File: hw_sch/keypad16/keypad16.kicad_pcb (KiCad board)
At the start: 2 copper layers, 70 x 100 mm, 174 parts, among them J1 Conn_01x04_Pin, J2 Conn_01x10_Pin, SW1 SW_Push, U1 MSP430FR2633IDAR, U2 TS5A23159RSE, U3 TS5A23159RSE, U4 TS5A23159RSE, U5 TS5A23159RSE, Y1 32.768KHz

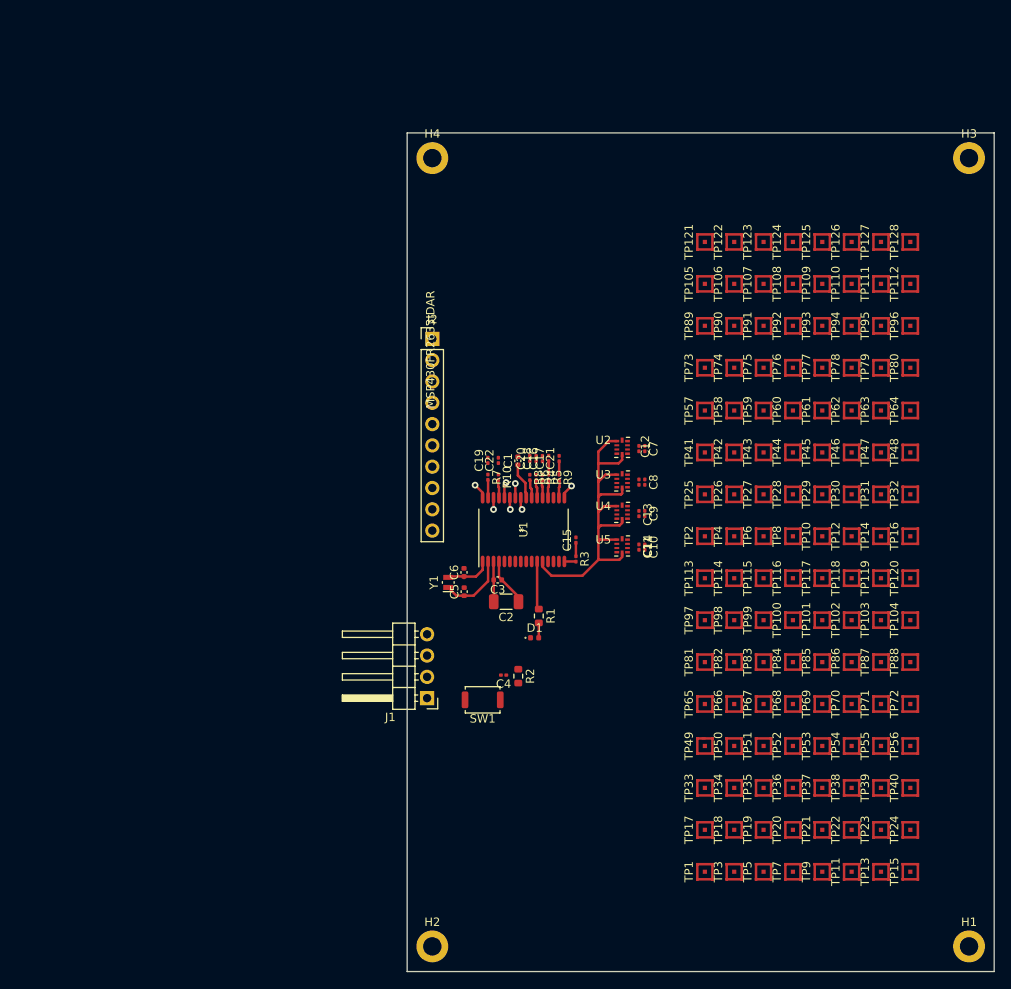
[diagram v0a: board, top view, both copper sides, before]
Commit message: finish keypad
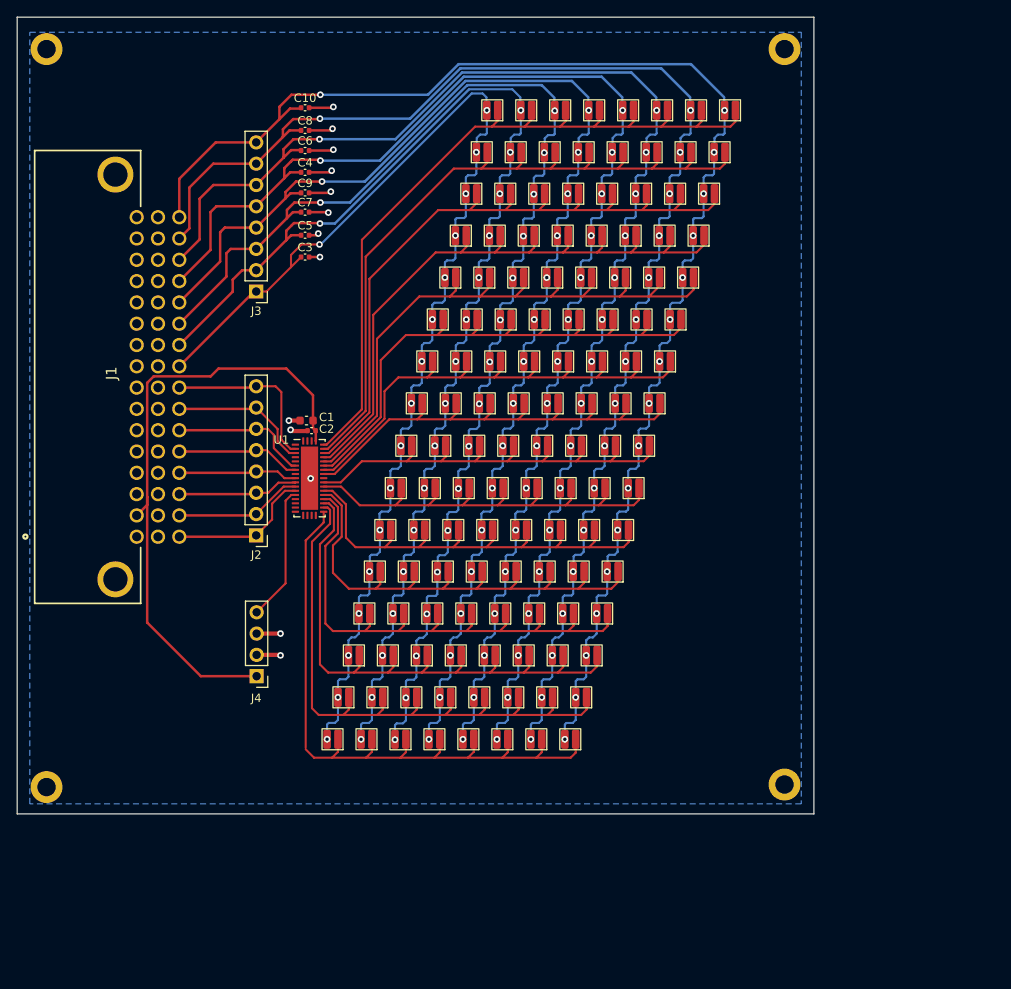
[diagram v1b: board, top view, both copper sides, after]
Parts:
- removed C11, C12, C13, C14: 0.1u, Capacitor_SMD:C_0201_0603Metric
- removed C15, C16, C17, C18, C19, C20, C21, C22: 68p, Capacitor_SMD:C_0201_0603Metric
- removed D1: LED, LED_SMD:LED_0402_1005Metric
- removed R1: 470, Resistor_SMD:R_0603_1608Metric
- removed R10, R3, R4, R5, R6, R7, R8, R9: 470, Resistor_SMD:R_0201_0603Metric
- removed R2: 47k, Resistor_SMD:R_0603_1608Metric
- removed SW1: SW_Push, Button_Switch_SMD:SW_Push_SPST_NO_Alps_SKRK
- removed U2, U3, U4, U5: TS5A23159RSE, Package_DFN_QFN:Texas_R-PUQFN-N10
- removed Y1: 32.768KHz, Crystal:Crystal_SMD_MicroCrystal_CM9V-T1A-2Pin_1.6x1.0mm
- added J3: Conn_01x08_Pin, Connector_PinHeader_2.54mm:PinHeader_1x08_P2.54mm_Vertical, F.Cu at (52.0, 68.9)
- added J4: Conn_01x04_Pin, Connector_PinHeader_2.54mm:PinHeader_1x04_P2.54mm_Vertical, F.Cu at (52.0, 114.8)
- C1: footprint Capacitor_SMD:C_0402_1005Metric -> Capacitor_SMD:C_0603_1608Metric
- C10, C7, C8, C9: value 1u -> 68p; footprint Capacitor_SMD:C_0201_0603Metric -> Capacitor_SMD:C_0402_1005Metric
- C2: value 10u -> 0.1u; footprint Capacitor_SMD:C_1206_3216Metric -> Capacitor_SMD:C_0402_1005Metric
- C3: value 0.1u -> 68p
- C4: value 1000n -> 68p; footprint Capacitor_SMD:C_0201_0603Metric -> Capacitor_SMD:C_0402_1005Metric
- C5, C6: value 22p -> 68p
- J1: value Conn_01x04_Pin -> 09231486921; footprint Connector_PinHeader_2.54mm:PinHeader_1x04_P2.54mm_Horizontal -> 09321:09231486921
- J2: value Conn_01x10_Pin -> Conn_01x08_Pin; footprint Connector_PinHeader_2.54mm:PinHeader_1x10_P2.54mm_Vertical -> Connector_PinHeader_2.54mm:PinHeader_1x08_P2.54mm_Vertical
- U1: value MSP430FR2633IDAR -> TS3L501ERUA; footprint footprints:MSP430FR2633IDAR -> Package_DFN_QFN:WQFN-42-1EP_3.5x9mm_P0.5mm_EP2.05x7.55mm
- moved TP72 74.0 mm to (108.5, 47.3), turned to 180 degrees
- moved TP120 72.2 mm to (84.2, 47.3), turned to 180 degrees
- moved TP88 72.2 mm to (100.4, 47.3), turned to 180 degrees
- moved TP104 71.6 mm to (92.3, 47.3), turned to 180 degrees
- moved TP71 68.6 mm to (107.2, 52.3), turned to 180 degrees
- moved TP119 66.9 mm to (83.0, 52.3), turned to 180 degrees
- moved TP87 66.7 mm to (99.2, 52.3), turned to 180 degrees
- moved TP56 66.5 mm to (74.0, 87.3), turned to 180 degrees
- moved C10 66.2 mm to (57.8, 47.0), turned to 0 degrees
- moved TP103 66.1 mm to (91.0, 52.3), turned to 180 degrees
- moved C4 64.5 mm to (57.8, 54.7), turned to 0 degrees
- moved TP70 63.2 mm to (106.0, 57.2), turned to 180 degrees
- moved TP40 63.0 mm to (82.0, 87.3), turned to 180 degrees
- moved TP55 62.0 mm to (72.7, 92.3), turned to 180 degrees
- moved TP118 61.7 mm to (81.7, 57.2), turned to 180 degrees
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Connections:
- C1 pad 1: /VREG -> +3V3
- C10 pad 1: +3V3 -> /FRX7
- C3 pad 1: +3V3 -> /FRX0
- C4 pad 1: /SPY_SWD_RST -> /FRX4
- C4 pad 2: /RESET -> GND
- C5 pad 1: /XIN -> /FRX1
- C6 pad 1: /XOUT -> /FRX5
- C7 pad 1: +3V3 -> /FRX2
- C8 pad 1: +3V3 -> /FRX6
- C9 pad 1: +3V3 -> /FRX3
- J2 pad 1: +3.3V -> /CAP0
- J2 pad 2: GND -> /CAP1
- J2 pad 3: GND -> /CAP2
- J2 pad 4: GND -> /CAP3
- J2 pad 5: /SPI_MOSI -> /CAP4
- J2 pad 6: /SPI_MISO -> /CAP5
- J2 pad 7: /SPI_CLK -> /CAP6
- J2 pad 8: /SPI_CE -> /CAP7
- TP1 pad 1: /Bus Switch/A0 -> /Bus Switch/B1
- TP1 pad 2: /FRX0 -> /FRX7
- TP10 pad 2: /FRX4 -> /FRX6
- TP100 pad 1: /Bus Switch/A6 -> /Bus Switch/A4
- TP101 pad 1: /Bus Switch/A6 -> /Bus Switch/B7
- TP101 pad 2: /FRX4 -> /FRX3
- TP102 pad 1: /Bus Switch/A6 -> /Bus Switch/B6
- TP102 pad 2: /FRX5 -> /FRX3
- TP103 pad 1: /Bus Switch/A6 -> /Bus Switch/A7
- TP103 pad 2: /FRX6 -> /FRX3
- TP104 pad 2: /FRX7 -> /FRX3
- TP105 pad 1: /Bus Switch/B6 -> /Bus Switch/B5
- TP105 pad 2: /FRX0 -> /FRX2
- TP106 pad 1: /Bus Switch/B6 -> /Bus Switch/B4
- TP106 pad 2: /FRX1 -> /FRX2
- TP107 pad 1: /Bus Switch/B6 -> /Bus Switch/A5
- TP108 pad 1: /Bus Switch/B6 -> /Bus Switch/A4
- TP108 pad 2: /FRX3 -> /FRX2
- TP109 pad 1: /Bus Switch/B6 -> /Bus Switch/B7
- TP109 pad 2: /FRX4 -> /FRX2
- TP11 pad 1: /Bus Switch/A0 -> /Bus Switch/A1
- TP11 pad 2: /FRX5 -> /FRX6
- TP110 pad 2: /FRX5 -> /FRX2
- TP111 pad 1: /Bus Switch/B6 -> /Bus Switch/A7
- TP111 pad 2: /FRX6 -> /FRX2
- TP112 pad 1: /Bus Switch/B6 -> /Bus Switch/A6
- TP112 pad 2: /FRX7 -> /FRX2
- TP113 pad 1: /Bus Switch/A7 -> /Bus Switch/B5
- TP113 pad 2: /FRX0 -> /FRX1
- TP114 pad 1: /Bus Switch/A7 -> /Bus Switch/B4
- TP115 pad 1: /Bus Switch/A7 -> /Bus Switch/A5
- TP115 pad 2: /FRX2 -> /FRX1
- TP116 pad 1: /Bus Switch/A7 -> /Bus Switch/A4
- TP116 pad 2: /FRX3 -> /FRX1
- TP117 pad 1: /Bus Switch/A7 -> /Bus Switch/B7
- TP117 pad 2: /FRX4 -> /FRX1
- TP118 pad 1: /Bus Switch/A7 -> /Bus Switch/B6
- TP118 pad 2: /FRX5 -> /FRX1
- TP119 pad 2: /FRX6 -> /FRX1
- TP12 pad 1: /Bus Switch/B0 -> /Bus Switch/A0
- TP12 pad 2: /FRX5 -> /FRX6
- TP120 pad 1: /Bus Switch/A7 -> /Bus Switch/A6
- TP120 pad 2: /FRX7 -> /FRX1
- TP121 pad 1: /Bus Switch/B7 -> /Bus Switch/B5
- TP122 pad 1: /Bus Switch/B7 -> /Bus Switch/B4
- TP122 pad 2: /FRX1 -> /FRX0
- TP123 pad 1: /Bus Switch/B7 -> /Bus Switch/A5
- TP123 pad 2: /FRX2 -> /FRX0
- TP124 pad 1: /Bus Switch/B7 -> /Bus Switch/A4
- TP124 pad 2: /FRX3 -> /FRX0
- TP125 pad 2: /FRX4 -> /FRX0
- TP126 pad 1: /Bus Switch/B7 -> /Bus Switch/B6
- TP126 pad 2: /FRX5 -> /FRX0
- TP127 pad 1: /Bus Switch/B7 -> /Bus Switch/A7
- TP127 pad 2: /FRX6 -> /FRX0
- TP128 pad 1: /Bus Switch/B7 -> /Bus Switch/A6
- TP128 pad 2: /FRX7 -> /FRX0
- TP13 pad 1: /Bus Switch/A0 -> /Bus Switch/B3
- TP14 pad 1: /Bus Switch/B0 -> /Bus Switch/B2
- TP15 pad 1: /Bus Switch/A0 -> /Bus Switch/A3
- TP15 pad 2: /FRX7 -> /FRX6
- TP16 pad 1: /Bus Switch/B0 -> /Bus Switch/A2
- TP16 pad 2: /FRX7 -> /FRX6
- TP17 pad 1: /Bus Switch/A1 -> /Bus Switch/B1
- TP17 pad 2: /FRX0 -> /FRX5
- TP18 pad 1: /Bus Switch/A1 -> /Bus Switch/B0
- TP18 pad 2: /FRX1 -> /FRX5
- TP19 pad 2: /FRX2 -> /FRX5
- TP2 pad 2: /FRX0 -> /FRX7
- TP20 pad 1: /Bus Switch/A1 -> /Bus Switch/A0
- TP20 pad 2: /FRX3 -> /FRX5
- TP21 pad 1: /Bus Switch/A1 -> /Bus Switch/B3
- TP21 pad 2: /FRX4 -> /FRX5
- TP22 pad 1: /Bus Switch/A1 -> /Bus Switch/B2
- TP23 pad 1: /Bus Switch/A1 -> /Bus Switch/A3
- TP23 pad 2: /FRX6 -> /FRX5
- TP24 pad 1: /Bus Switch/A1 -> /Bus Switch/A2
- TP24 pad 2: /FRX7 -> /FRX5
- TP25 pad 2: /FRX0 -> /FRX4
- TP26 pad 1: /Bus Switch/B1 -> /Bus Switch/B0
- TP26 pad 2: /FRX1 -> /FRX4
- TP27 pad 1: /Bus Switch/B1 -> /Bus Switch/A1
- TP27 pad 2: /FRX2 -> /FRX4
- TP28 pad 1: /Bus Switch/B1 -> /Bus Switch/A0
- TP28 pad 2: /FRX3 -> /FRX4
- TP29 pad 1: /Bus Switch/B1 -> /Bus Switch/B3
- TP3 pad 1: /Bus Switch/A0 -> /Bus Switch/A1
- TP3 pad 2: /FRX1 -> /FRX7
- TP30 pad 1: /Bus Switch/B1 -> /Bus Switch/B2
- TP30 pad 2: /FRX5 -> /FRX4
- TP31 pad 1: /Bus Switch/B1 -> /Bus Switch/A3
- TP31 pad 2: /FRX6 -> /FRX4
- TP32 pad 1: /Bus Switch/B1 -> /Bus Switch/A2
- TP32 pad 2: /FRX7 -> /FRX4
- TP33 pad 1: /Bus Switch/A2 -> /Bus Switch/B1
- TP33 pad 2: /FRX0 -> /FRX3
- TP34 pad 1: /Bus Switch/A2 -> /Bus Switch/B0
- TP34 pad 2: /FRX1 -> /FRX3
- TP35 pad 1: /Bus Switch/A2 -> /Bus Switch/A1
- TP35 pad 2: /FRX2 -> /FRX3
- TP36 pad 1: /Bus Switch/A2 -> /Bus Switch/A0
- TP37 pad 1: /Bus Switch/A2 -> /Bus Switch/B3
- TP37 pad 2: /FRX4 -> /FRX3
- TP38 pad 1: /Bus Switch/A2 -> /Bus Switch/B2
- TP38 pad 2: /FRX5 -> /FRX3
- TP39 pad 1: /Bus Switch/A2 -> /Bus Switch/A3
- TP39 pad 2: /FRX6 -> /FRX3
- TP4 pad 1: /Bus Switch/B0 -> /Bus Switch/A0
- TP4 pad 2: /FRX1 -> /FRX7
- TP40 pad 2: /FRX7 -> /FRX3
- TP41 pad 1: /Bus Switch/B2 -> /Bus Switch/B1
- TP41 pad 2: /FRX0 -> /FRX2
- TP42 pad 1: /Bus Switch/B2 -> /Bus Switch/B0
- TP42 pad 2: /FRX1 -> /FRX2
- TP43 pad 1: /Bus Switch/B2 -> /Bus Switch/A1
- TP44 pad 1: /Bus Switch/B2 -> /Bus Switch/A0
- TP44 pad 2: /FRX3 -> /FRX2
- TP45 pad 1: /Bus Switch/B2 -> /Bus Switch/B3
- TP45 pad 2: /FRX4 -> /FRX2
- TP46 pad 2: /FRX5 -> /FRX2
- TP47 pad 1: /Bus Switch/B2 -> /Bus Switch/A3
- TP47 pad 2: /FRX6 -> /FRX2
- TP48 pad 1: /Bus Switch/B2 -> /Bus Switch/A2
- TP48 pad 2: /FRX7 -> /FRX2
- TP49 pad 1: /Bus Switch/A3 -> /Bus Switch/B1
- TP49 pad 2: /FRX0 -> /FRX1
- TP5 pad 1: /Bus Switch/A0 -> /Bus Switch/B3
- TP5 pad 2: /FRX2 -> /FRX7
- TP50 pad 1: /Bus Switch/A3 -> /Bus Switch/B0
- TP51 pad 1: /Bus Switch/A3 -> /Bus Switch/A1
- TP51 pad 2: /FRX2 -> /FRX1
- TP52 pad 1: /Bus Switch/A3 -> /Bus Switch/A0
- TP52 pad 2: /FRX3 -> /FRX1
- TP53 pad 1: /Bus Switch/A3 -> /Bus Switch/B3
- TP53 pad 2: /FRX4 -> /FRX1
- TP54 pad 1: /Bus Switch/A3 -> /Bus Switch/B2
- TP54 pad 2: /FRX5 -> /FRX1
- TP55 pad 2: /FRX6 -> /FRX1
- TP56 pad 1: /Bus Switch/A3 -> /Bus Switch/A2
- TP56 pad 2: /FRX7 -> /FRX1
- TP57 pad 1: /Bus Switch/B3 -> /Bus Switch/B1
- TP58 pad 1: /Bus Switch/B3 -> /Bus Switch/B0
- TP58 pad 2: /FRX1 -> /FRX0
- TP59 pad 1: /Bus Switch/B3 -> /Bus Switch/A1
- TP59 pad 2: /FRX2 -> /FRX0
- TP6 pad 1: /Bus Switch/B0 -> /Bus Switch/B2
- TP6 pad 2: /FRX2 -> /FRX7
- TP60 pad 1: /Bus Switch/B3 -> /Bus Switch/A0
- TP60 pad 2: /FRX3 -> /FRX0
- TP61 pad 2: /FRX4 -> /FRX0
- TP62 pad 1: /Bus Switch/B3 -> /Bus Switch/B2
- TP62 pad 2: /FRX5 -> /FRX0
- TP63 pad 1: /Bus Switch/B3 -> /Bus Switch/A3
- TP63 pad 2: /FRX6 -> /FRX0
- TP64 pad 1: /Bus Switch/B3 -> /Bus Switch/A2
- TP64 pad 2: /FRX7 -> /FRX0
- TP65 pad 1: /Bus Switch/A4 -> /Bus Switch/B5
- TP65 pad 2: /FRX0 -> /FRX7
- TP66 pad 1: /Bus Switch/A4 -> /Bus Switch/B4
- TP66 pad 2: /FRX1 -> /FRX7
- TP67 pad 1: /Bus Switch/A4 -> /Bus Switch/A5
- TP67 pad 2: /FRX2 -> /FRX7
- TP68 pad 2: /FRX3 -> /FRX7
- TP69 pad 1: /Bus Switch/A4 -> /Bus Switch/B7
- TP69 pad 2: /FRX4 -> /FRX7
- TP7 pad 1: /Bus Switch/A0 -> /Bus Switch/A3
- TP7 pad 2: /FRX3 -> /FRX7
- TP70 pad 1: /Bus Switch/A4 -> /Bus Switch/B6
- TP70 pad 2: /FRX5 -> /FRX7
- TP71 pad 1: /Bus Switch/A4 -> /Bus Switch/A7
- TP71 pad 2: /FRX6 -> /FRX7
- TP72 pad 1: /Bus Switch/A4 -> /Bus Switch/A6
- TP73 pad 1: /Bus Switch/B4 -> /Bus Switch/B5
- TP73 pad 2: /FRX0 -> /FRX6
- TP74 pad 2: /FRX1 -> /FRX6
- TP75 pad 1: /Bus Switch/B4 -> /Bus Switch/A5
- TP75 pad 2: /FRX2 -> /FRX6
- TP76 pad 1: /Bus Switch/B4 -> /Bus Switch/A4
- TP76 pad 2: /FRX3 -> /FRX6
- TP77 pad 1: /Bus Switch/B4 -> /Bus Switch/B7
- TP77 pad 2: /FRX4 -> /FRX6
- TP78 pad 1: /Bus Switch/B4 -> /Bus Switch/B6
- TP78 pad 2: /FRX5 -> /FRX6
- TP79 pad 1: /Bus Switch/B4 -> /Bus Switch/A7
- TP8 pad 1: /Bus Switch/B0 -> /Bus Switch/A2
- TP8 pad 2: /FRX3 -> /FRX7
- TP80 pad 1: /Bus Switch/B4 -> /Bus Switch/A6
- TP80 pad 2: /FRX7 -> /FRX6
- TP81 pad 1: /Bus Switch/A5 -> /Bus Switch/B5
- TP81 pad 2: /FRX0 -> /FRX5
- TP82 pad 1: /Bus Switch/A5 -> /Bus Switch/B4
- TP82 pad 2: /FRX1 -> /FRX5
- TP83 pad 2: /FRX2 -> /FRX5
- TP84 pad 1: /Bus Switch/A5 -> /Bus Switch/A4
- TP84 pad 2: /FRX3 -> /FRX5
- TP85 pad 1: /Bus Switch/A5 -> /Bus Switch/B7
- TP85 pad 2: /FRX4 -> /FRX5
- TP86 pad 1: /Bus Switch/A5 -> /Bus Switch/B6
- TP87 pad 1: /Bus Switch/A5 -> /Bus Switch/A7
- TP87 pad 2: /FRX6 -> /FRX5
- TP88 pad 1: /Bus Switch/A5 -> /Bus Switch/A6
- TP88 pad 2: /FRX7 -> /FRX5
- TP89 pad 2: /FRX0 -> /FRX4
- TP9 pad 1: /Bus Switch/A0 -> /Bus Switch/B1
- TP9 pad 2: /FRX4 -> /FRX6
- TP90 pad 1: /Bus Switch/B5 -> /Bus Switch/B4
- TP90 pad 2: /FRX1 -> /FRX4
- TP91 pad 1: /Bus Switch/B5 -> /Bus Switch/A5
- TP91 pad 2: /FRX2 -> /FRX4
- TP92 pad 1: /Bus Switch/B5 -> /Bus Switch/A4
- TP92 pad 2: /FRX3 -> /FRX4
- TP93 pad 1: /Bus Switch/B5 -> /Bus Switch/B7
- TP94 pad 1: /Bus Switch/B5 -> /Bus Switch/B6
- TP94 pad 2: /FRX5 -> /FRX4
- TP95 pad 1: /Bus Switch/B5 -> /Bus Switch/A7
- TP95 pad 2: /FRX6 -> /FRX4
- TP96 pad 1: /Bus Switch/B5 -> /Bus Switch/A6
- TP96 pad 2: /FRX7 -> /FRX4
- TP97 pad 1: /Bus Switch/A6 -> /Bus Switch/B5
- TP97 pad 2: /FRX0 -> /FRX3
- TP98 pad 1: /Bus Switch/A6 -> /Bus Switch/B4
- TP98 pad 2: /FRX1 -> /FRX3
- TP99 pad 1: /Bus Switch/A6 -> /Bus Switch/A5
- TP99 pad 2: /FRX2 -> /FRX3
- U1 pad 1: /XOUT -> unconnected-(U1F-VDD-Pad1)
- U1 pad 10: /SPI_CE -> /CAP2
- U1 pad 11: /STATUS_LED -> /CAP1
- U1 pad 12: /CAP_SW -> /CAP0
- U1 pad 13: unconnected-(U1-P1-2_UCB0SIMO_UCB0SDA_TA0-2_A2_VEREF--Pad13) -> /CAP_SW
- U1 pad 16: /RX0 -> unconnected-(U1E-LED_A1-Pad16)
- U1 pad 17: /CAP0 -> unconnected-(U1E-LED_B0-Pad17)
- U1 pad 18: /RX3 -> unconnected-(U1E-LED_B1-Pad18)
- U1 pad 19: /CAP1 -> unconnected-(U1E-LED_C0-Pad19)
- U1 pad 2: /XIN -> /CAP7
- U1 pad 20: /RX1 -> unconnected-(U1E-LED_C1-Pad20)
- U1 pad 21: /RX4 -> unconnected-(U1F-VDD-Pad21)
- U1 pad 22: /RX5 -> /Bus Switch/B1
- U1 pad 23: /RX6 -> /Bus Switch/B0
- U1 pad 24: /VREG -> /Bus Switch/A1
- U1 pad 25: /CAP2 -> /Bus Switch/A0
- U1 pad 26: /CAP3 -> /Bus Switch/B3
- U1 pad 27: /CAP4 -> /Bus Switch/B2
- U1 pad 28: /CAP5 -> /Bus Switch/A3
- U1 pad 29: /RX7 -> /Bus Switch/A2
- U1 pad 3: GND -> /CAP6
- U1 pad 30: /CAP6 -> unconnected-(U1F-VDD-Pad30)
- U1 pad 31: /RX2 -> /Bus Switch/B5
- U1 pad 32: /CAP7 -> /Bus Switch/B4
- U1 pad 4: +3V3 -> unconnected-(U1F-VDD-Pad4)
- U1 pad 5: /SPY_SWD_RST -> unconnected-(U1F-PD-Pad5)
- U1 pad 6: /SPY_CLK -> /CAP5
- U1 pad 7: /SPI_MOSI -> /CAP4
- U1 pad 8: /SPI_MISO -> unconnected-(U1F-VDD-Pad8)
- U1 pad 9: /SPI_CLK -> /CAP3
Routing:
- net /FRX7: track 0.00 -> 171.8 mm, vias 0 -> 17
- net /FRX6: track 0.00 -> 167.6 mm, vias 0 -> 17
- net /FRX5: track 0.00 -> 164.2 mm, vias 0 -> 17
- net /FRX4: track 0.00 -> 160.6 mm, vias 0 -> 17
- net /FRX3: track 1.61 -> 156.0 mm, vias 0 -> 17
- net /FRX2: track 0.00 -> 152.2 mm, vias 0 -> 17
- net /FRX1: track 1.61 -> 148.1 mm, vias 0 -> 17
- net /FRX0: track 1.61 -> 143.5 mm, vias 0 -> 17
- net /Bus Switch/A6: track 0.00 -> 93.9 mm
- net /Bus Switch/A7: track 0.00 -> 89.5 mm
- net /Bus Switch/B6: track 0.00 -> 85.1 mm
- net /Bus Switch/B7: track 0.00 -> 79.8 mm
- net /Bus Switch/B1: track 0.00 -> 79.2 mm
- net /Bus Switch/A4: track 0.00 -> 78.0 mm
- net /Bus Switch/B0: track 0.00 -> 76.8 mm
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- added copper zone on B.Cu, net GND
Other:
- board size 70 x 100 mm -> 95 x 95 mm
